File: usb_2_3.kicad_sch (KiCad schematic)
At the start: 20 parts, among them J4 USB3_A_Stacked, J5 USB_A_Stacked, U3 D3V3XA4B10LP, U4 D3V3XA4B10LP, U5 D3V3XA4B10LP

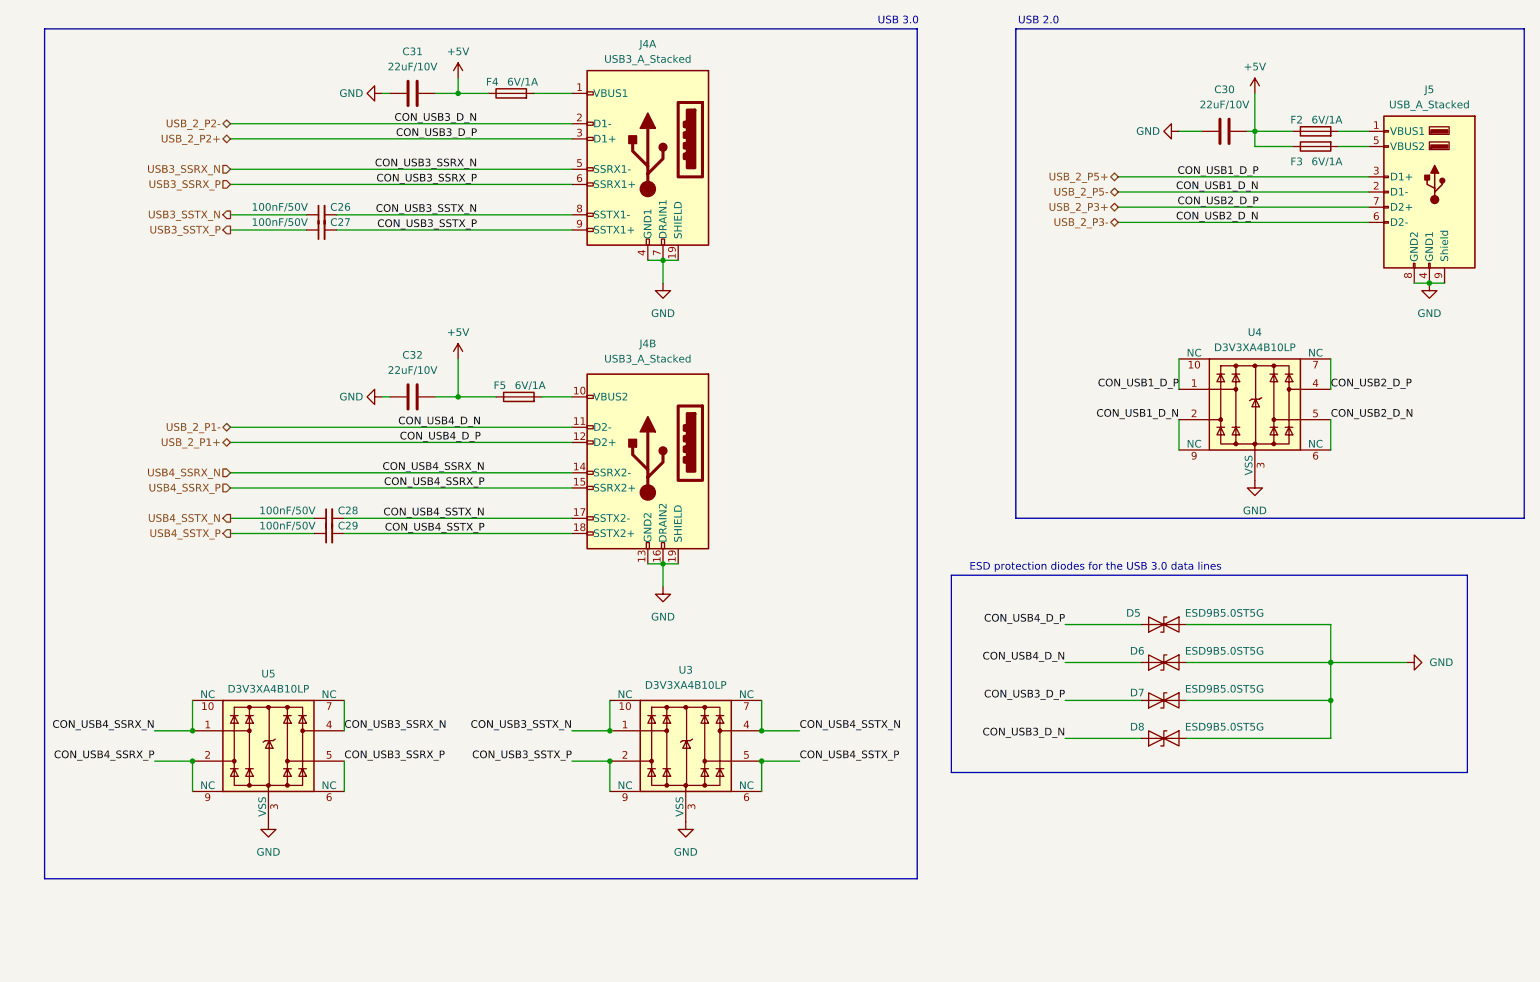
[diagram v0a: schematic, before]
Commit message: added reference design and finished routing
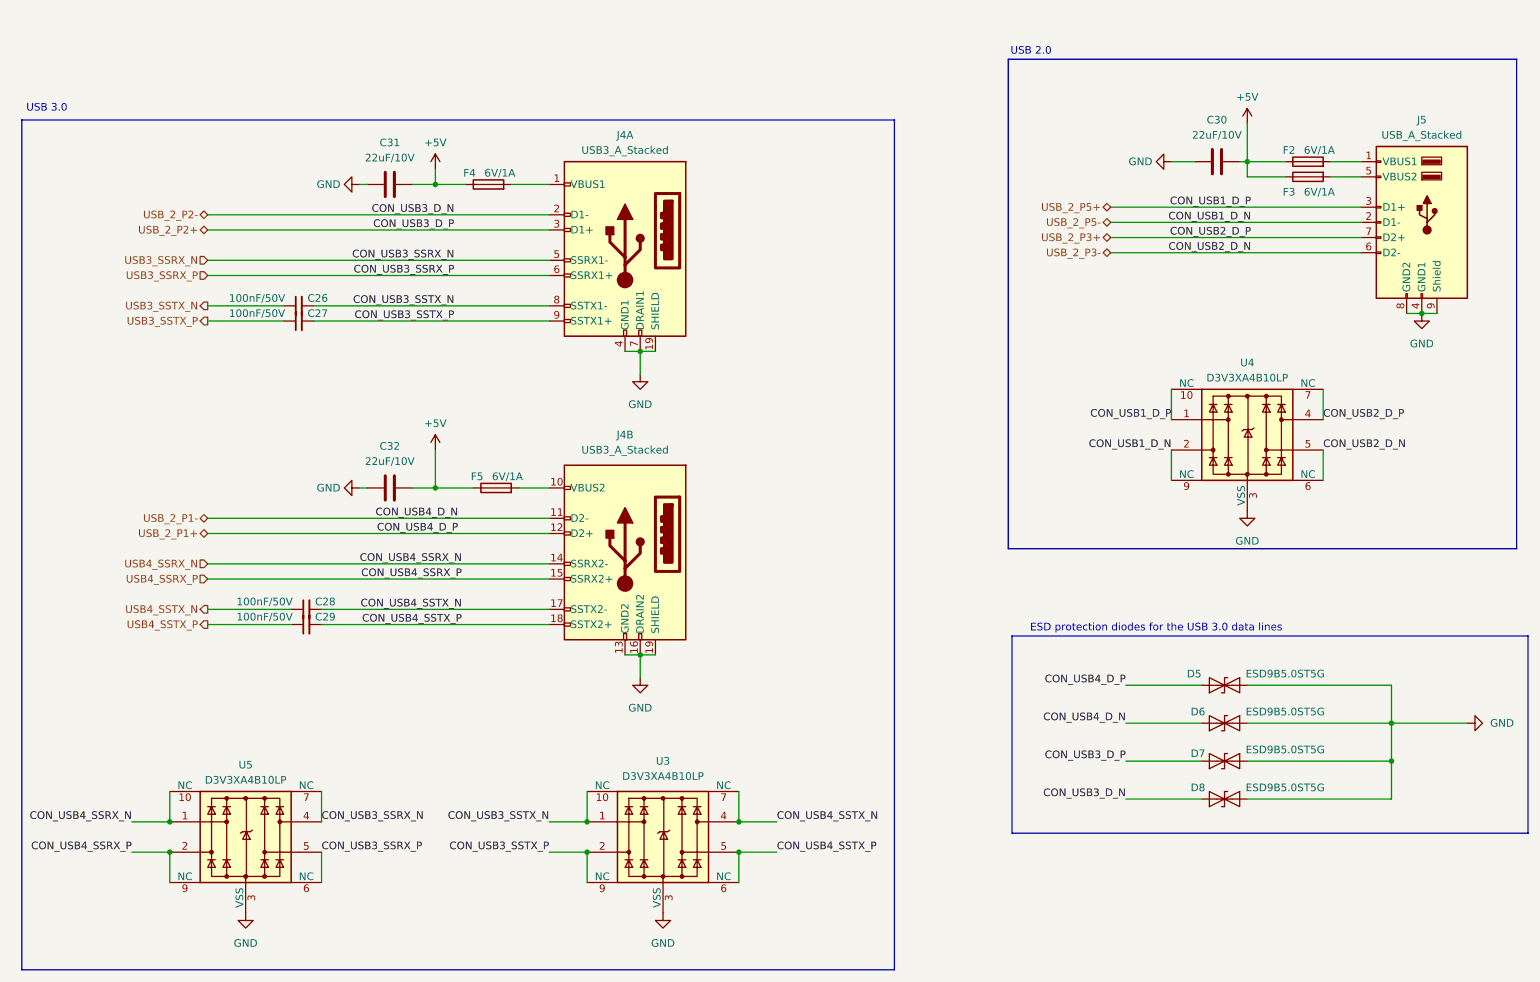
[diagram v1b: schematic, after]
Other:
- moved on the sheet: C26, C27, C28, C29, C30, C31, C32, D5, D6, D7, D8, F2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
